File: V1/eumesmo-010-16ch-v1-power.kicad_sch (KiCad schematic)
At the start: 56 parts, among them J6 250-202, J7 USB_C_Receptacle_USB2.0, Q1 WPM2015-3/TR, Q2 MMUN2211LT3G, U1 TX4138, U11 L78L12, U12 L78L05, U2 SY8089A1AAC, U9 B2415S-1WR3

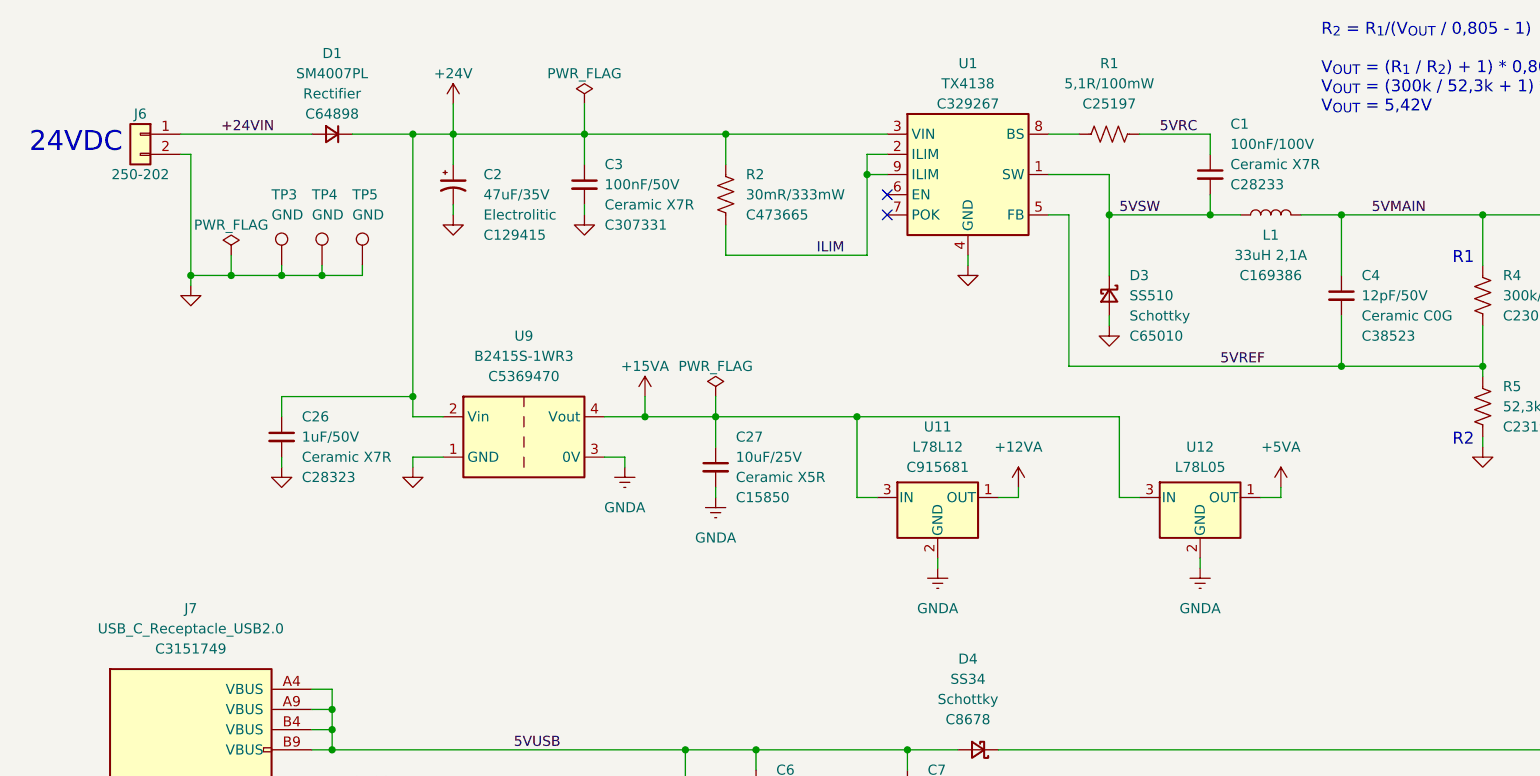
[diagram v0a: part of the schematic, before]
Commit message: Development
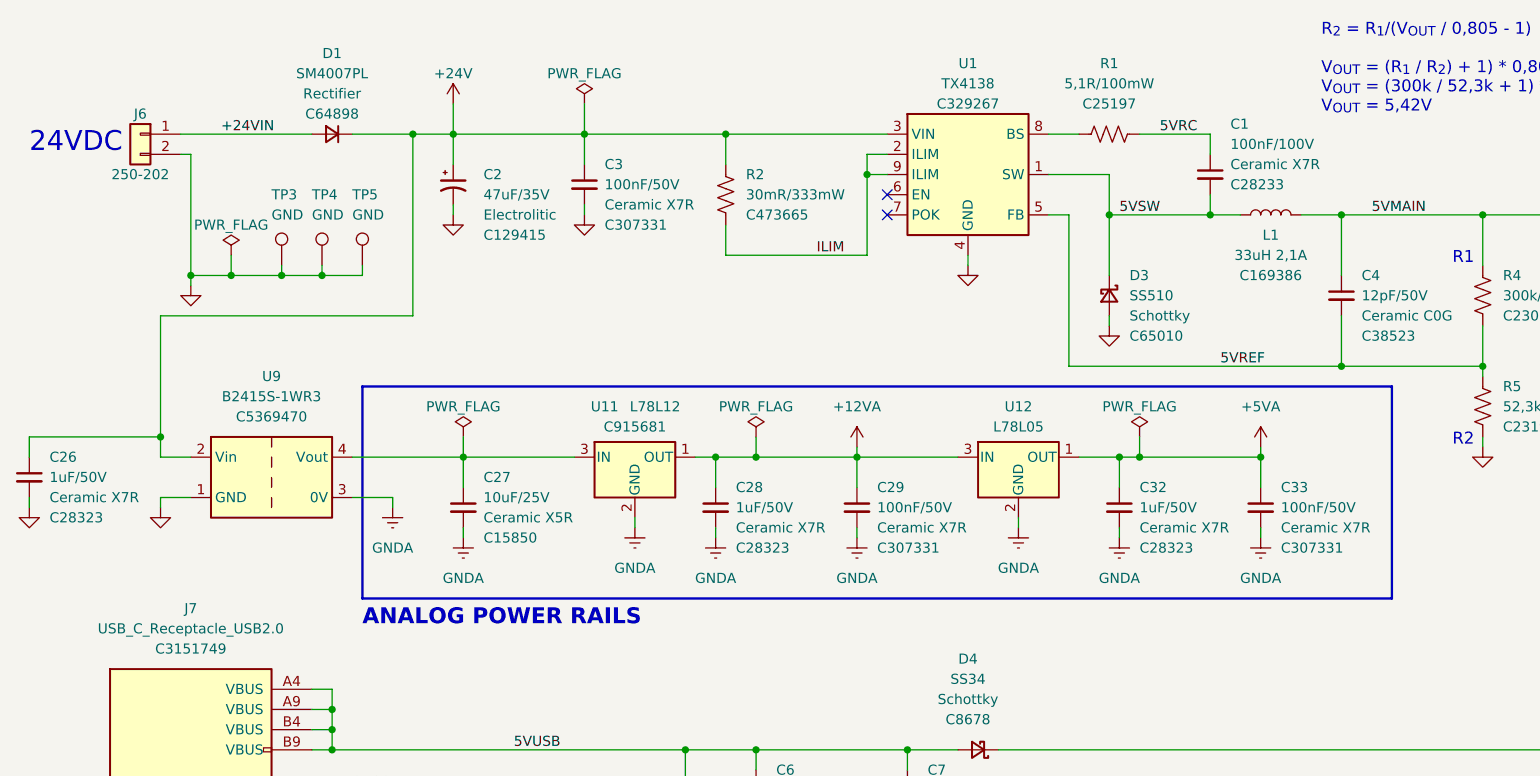
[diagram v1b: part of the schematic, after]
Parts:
- added C28, C32: 1uF/50V, Tales:C_0805_2012Metric, symbol Device:C_Small
- added C29, C33: 100nF/50V, Tales:C_0402_1005Metric, symbol Device:C_Small
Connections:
- net +12VA: now also U12.3 (IN), C28.1, C29.1
- net +5VA: now also C32.1, C33.1
- net GNDA: now also C28.2, C29.2, C32.2, C33.2
- net +15VA: no longer names the net of C27.1, U11.3 (IN), U9.4 (Vout)
- net +15VA: no longer U12.3 (IN)
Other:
- note added: "ANALOG POWER RAILS"
- moved on the sheet: C26, C27, U11, U12, U9
